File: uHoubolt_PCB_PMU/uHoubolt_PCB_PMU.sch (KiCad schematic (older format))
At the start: 44 parts, among them J1 Conn_01x04, J2 Conn_01x02, J3 Conn_01x04, Q2 Si7141DP, SW1 SW_Push_SPDT, SW2 SW_Push_SPDT, U1 INA226, U2 MAX1873SEEE

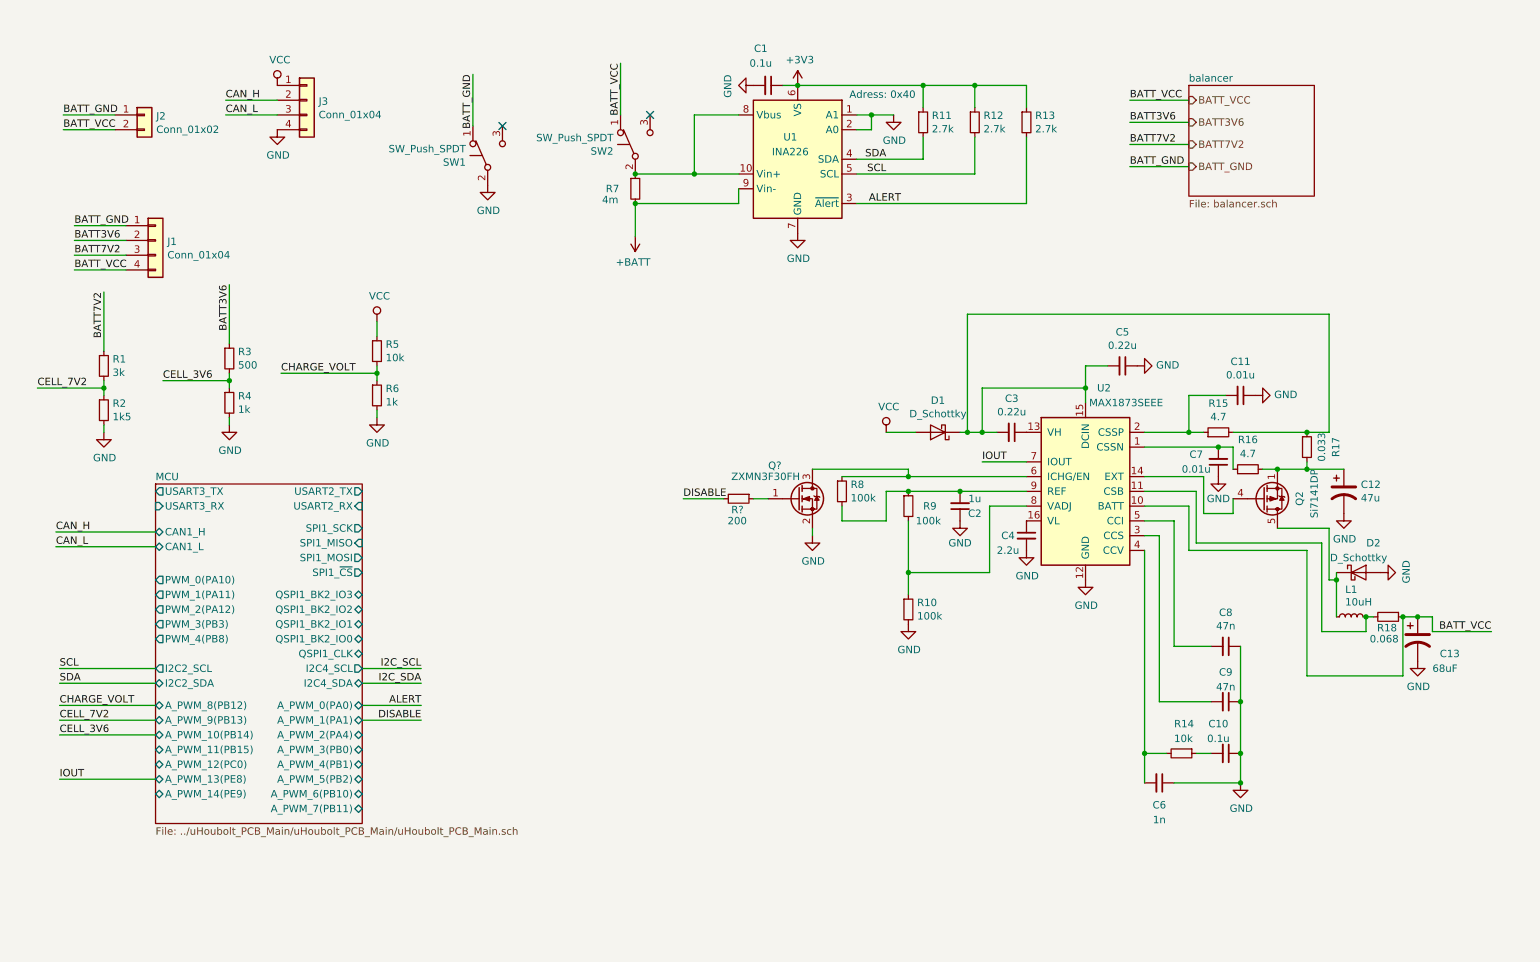
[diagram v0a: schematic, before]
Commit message: Add descriptions
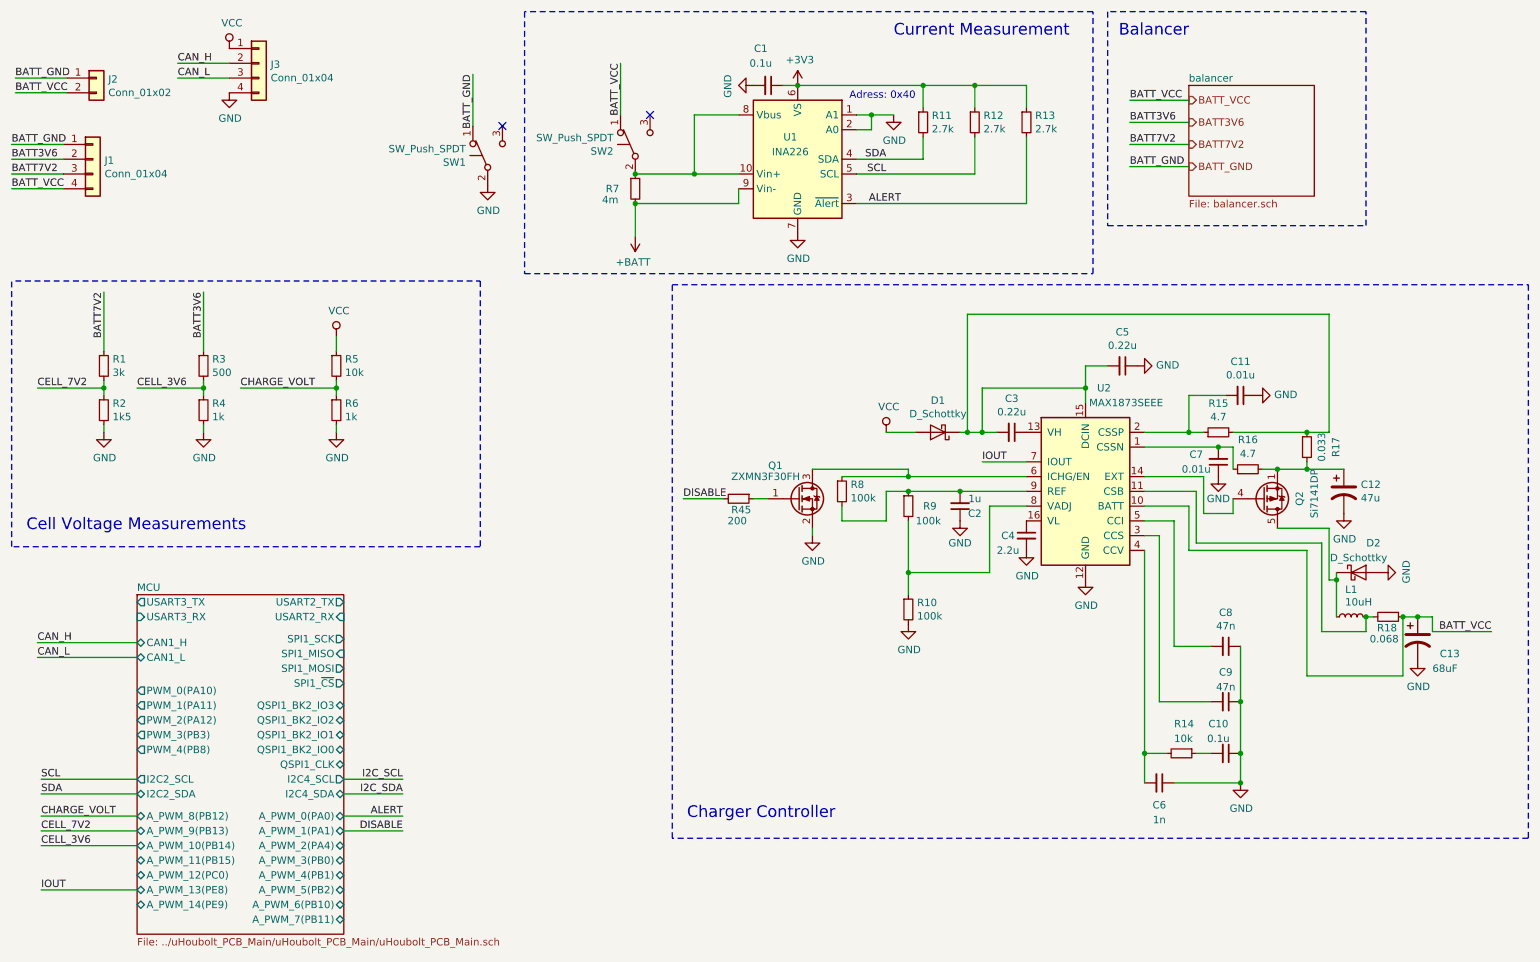
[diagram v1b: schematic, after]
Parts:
- gave numbers to parts that had none: 2
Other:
- note added: "Balancer"
- note added: "Cell Voltage Measurements\n"
- note added: "Charger Controller"
- note added: "Current Measurement"
- moved on the sheet: J1, J2, J3, R3, R4, R5, R6
